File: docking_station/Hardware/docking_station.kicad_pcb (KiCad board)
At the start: 2 copper layers, 115 x 43 mm, 108 parts, among them IC1 VOM1271T, IC2 VOM1271T, IC3 VOM1271T, IC4 VOM1271T, IC5 VOM1271T, J1 SUPPLY+, J2 SUPPLY-, J3 Conn_01x05_Pin, J4 XT60, J5 WAGO, K1 RELPOL R40N-3021-85-1024, Q1 SIDR392DP-T1-GE3, Q10 2N7002K, Q11 2N7002K, Q12 2N7002K, Q13 2N7002K, Q2 SIDR392DP-T1-GE3, Q3 SIDR392DP-T1-GE3, Q4 SIDR392DP-T1-GE3, Q5 SIDR392DP-T1-GE3, Q6 SIDR392DP-T1-GE3, Q7 SIDR392DP-T1-GE3, Q8 SIDR392DP-T1-GE3, Q9 SIDR392DP-T1-GE3, U1 LTC4357MS8, U2 L78L05AB, U3 ACS712xLCTR-20A, U4 LMV321IYLT, U5 MCP6561T-E/OT, U6 MCP6561T-E/OT, U7 MCP6561T-E/OT

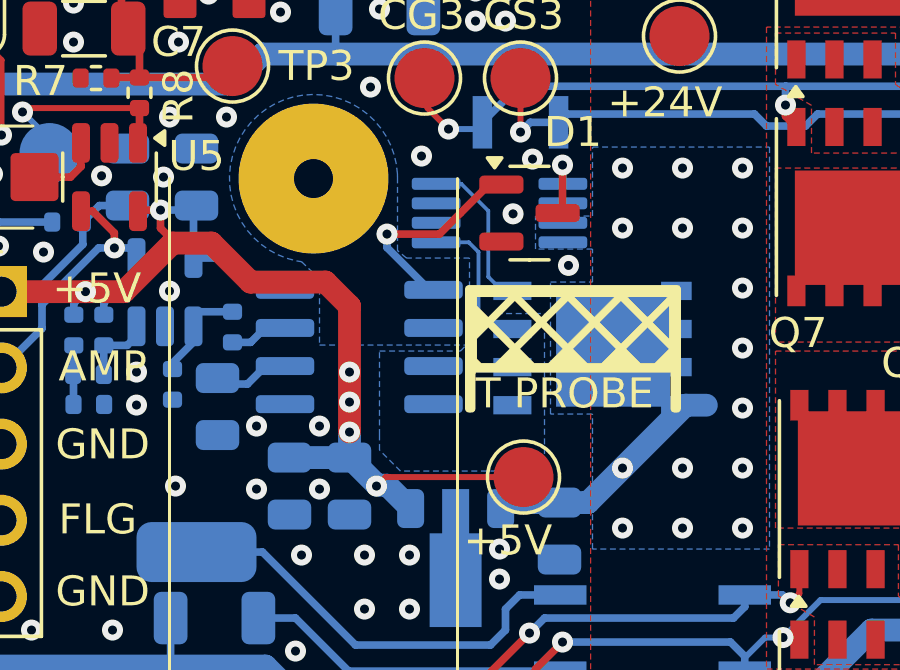
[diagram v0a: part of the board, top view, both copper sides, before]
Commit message: gaining_a_level_of_exhaustion_xd
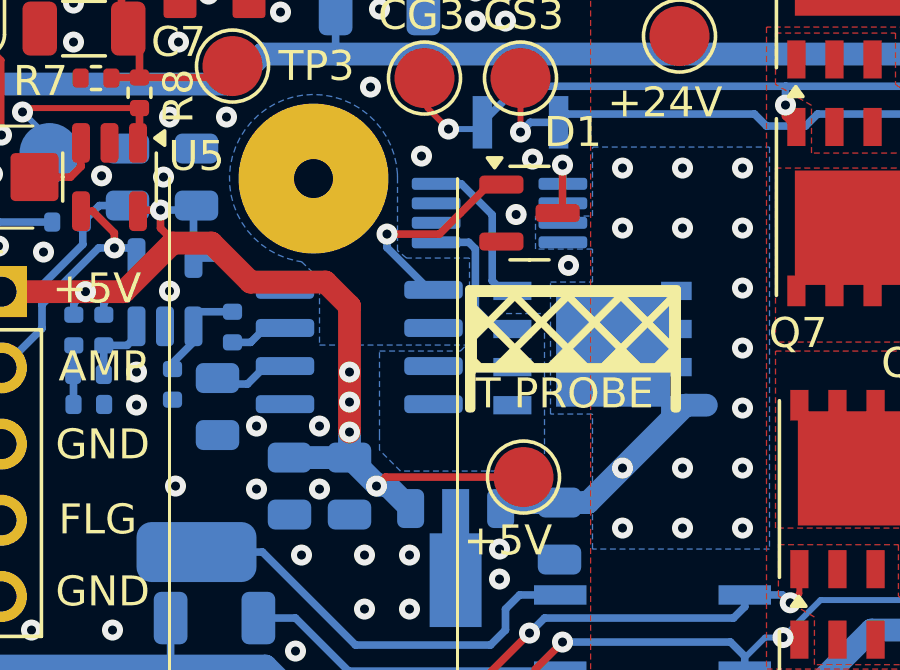
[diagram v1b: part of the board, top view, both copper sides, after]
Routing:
- net SENSE-: track 4.35 -> 4.91 mm
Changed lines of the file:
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@@
 	)
 	(via
-		(at 159.751712 98.725856)
+		(at 159.854421 98.748132)
 		(size 0.7)
 		(drill 0.3)
@@
 		(start 155.2 107.8)
 		(end 155.5 107.5)
-		(width 0.2)
+		(width 0.254)
 		(layer "F.Cu")
 		(net 3)
@@
 		(start 155.5 107.5)
 		(end 160.1 107.5)
-		(width 0.2)
+		(width 0.254)
 		(layer "F.Cu")
 		(net 3)
@@
 	)
 	(segment
-		(start 155.2 107.8)
-		(end 155.5875 107.8)
-		(width 0.127)
-		(layer "B.Cu")
-		(net 3)
-	)
-	(segment
 		(start 145.41 99)
 		(end 145.41 99.747948)
@@
 	)
 	(segment
-		(start 158.6 100)
-		(end 158.6 102)
-		(width 0.127)
+		(start 159.165 102.565)
+		(end 159.73 102.565)
+		(width 0.254)
 		(layer "B.Cu")
 		(net 31)
 	)
 	(segment
-		(start 158.275 99.675)
-		(end 158.6 100)
-		(width 0.127)
+		(start 158.496 99.896)
+		(end 158.496 101.896)
+		(width 0.254)
 		(layer "B.Cu")
 		(net 31)
 	)
 	(segment
-		(start 158.6 102)
-		(end 159.165 102.565)
-		(width 0.127)
+		(start 157.1875 99.675)
+		(end 158.275 99.675)
+		(width 0.254)
 		(layer "B.Cu")
 		(net 31)
 	)
 	(segment
-		(start 157.1875 99.675)
-		(end 158.275 99.675)
-		(width 0.127)
+		(start 158.275 99.675)
+		(end 158.496 99.896)
+		(width 0.254)
 		(layer "B.Cu")
 		(net 31)
 	)
 	(segment
-		(start 158.927 100.827)
-		(end 159.395 101.295)
-		(width 0.127)
+		(start 158.496 101.896)
+		(end 159.165 102.565)
+		(width 0.254)
 		(layer "B.Cu")
-		(net 32)
+		(net 31)
 	)
 	(segment
-		(start 157.1875 97.725)
-		(end 158.025 97.725)
-		(width 0.127)
+		(start 159.395 101.295)
+		(end 159.73 101.295)
+		(width 0.254)
 		(layer "B.Cu")
 		(net 32)
 	)
 	(segment
-		(start 159.395 101.295)
-		(end 159.73 101.295)
-		(width 0.127)
+		(start 159.0572 98.7572)
+		(end 159.0572 100.9572)
+		(width 0.254)
 		(layer "B.Cu")
 		(net 32)
@@
 	(segment
 		(start 158.025 97.725)
-		(end 158.927 98.627)
-		(width 0.127)
+		(end 159.0572 98.7572)
+		(width 0.254)
+		(layer "B.Cu")
+		(net 32)
+	)
+	(segment
+		(start 159.0572 100.9572)
+		(end 159.395 101.295)
+		(width 0.254)
 		(layer "B.Cu")
 		(net 32)
 	)
 	(segment
-		(start 158.927 98.627)
-		(end 158.927 100.827)
-		(width 0.127)
+		(start 157.1875 97.725)
+		(end 158.025 97.725)
+		(width 0.254)
 		(layer "B.Cu")
 		(net 32)
